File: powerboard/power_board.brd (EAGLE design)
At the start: 149.9 x 86.4 mm, 100 parts, among them Q1 IPP80P03P4L04AKSA1, U1 UWQ-12/20-T48NBS-C, U2 UWE-5/20-Q48NB-C, U3 UWE-3.3/30-Q48NB-C

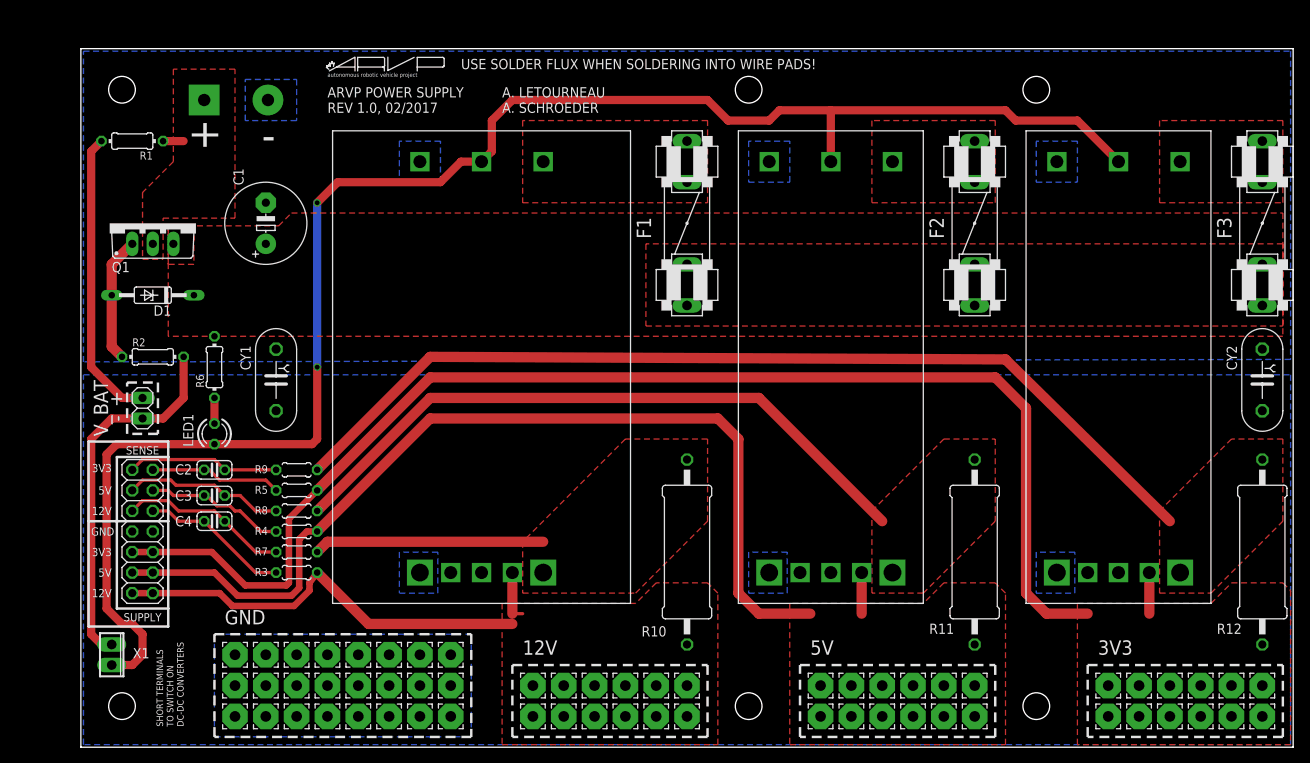
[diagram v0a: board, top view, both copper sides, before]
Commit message: fixed the branch
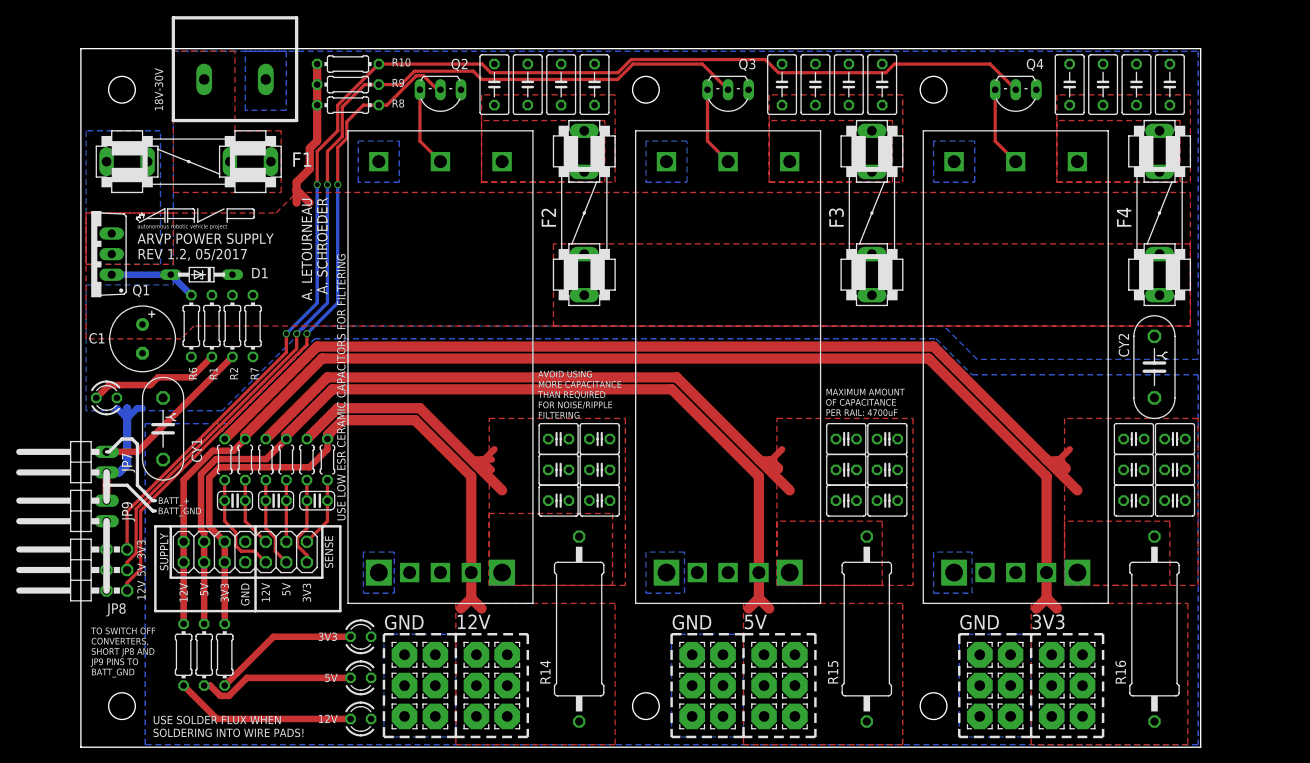
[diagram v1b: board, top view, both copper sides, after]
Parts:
- removed P$1: AND_PWR, ARVP:AND_PWR
- removed PAD37, PAD38, PAD39, PAD40, PAD41, PAD42, PAD43, PAD44, PAD45, PAD46, PAD47, PAD48, PAD49, PAD50, PAD51, PAD52, PAD53, PAD54, PAD55, PAD56, PAD57, PAD58, PAD59, PAD60: WIREPAD3,17/1,3, wirepad:3,17/1,3
- removed U3: UWE-3.3/30-Q48NB-C, New Power Board Library:UWE-100-120W
- removed X1: (no value), con-phoenix-254:2POL254
- added C10, C11, C12, C13, C14, C15, C16, C5, C6, C7, C8, C9: (no value), rcl:C050-035X075
- added C17, C18, C19, C20, C21, C22, C23, C24, C25, C26, C27, C28, C29, C30, C31, C32, C33, C34: (no value), rcl:C025-040X050
- added F4: (no value), special:FUSE1
- added JP10: (no value), pinhead:2X07
- added JP9: (no value), pinhead:1X02/90
- added LED2, LED3, LED4: (no value), led:LED3MM
- added Q2, Q3, Q4: 2N4401TFR, New Power Board Library:TO92-EBC
- added R13: 10, rcl:0204/5
- added R14, R15, R16: 0.004, rcl:0617/22
- added R17, R18, R19: 36k, resistor:0204/7
- added T1: 2_POS_TERMINAL, New Power Board Library:PHOENIX_CONTACT_MKDS_5/2-7.62
- added U4: UWE-12/10-Q48NB-C, New Power Board Library:UWE-100-120W
- C1: value (none) -> 100u; device rcl:E5-10,5 -> rcl:E3,5-8
- D1: value (none) -> BZV10; device diode:DO35Z10 -> diode:DO34Z7
- JP7: device pinhead:1X02 -> pinhead:1X02/90
- JP8: device pinhead:2X07 -> pinhead:2X03/90
- R1: value 1k -> 36k
- R10: value 0.004 -> 10k; device rcl:0617/22 -> resistor:0204/7
- R11, R12: value 0.004 -> 10; device rcl:0617/22 -> rcl:0204/5
- R2: value 100k -> 4.7k
- R6: value 1k -> 2k
- R7: value 10 -> 4.7k; device rcl:0204/5 -> resistor:0204/7
- R8, R9: value 10 -> 10k; device rcl:0204/5 -> resistor:0204/7
- U$1: device frames:DINA5_L -> frames:FRAME_A_L
- U1: value UWQ-12/20-T48NBS-C -> UWE-5/20-Q48NB-C; device New Power Board Library:UWQ-12/20-T48 -> New Power Board Library:UWE-100-120W
- U2: value UWE-5/20-Q48NB-C -> UWE-3.3/30-Q48NB-C
- moved R12 121.2 mm to (54.6, 26.7), turned to 90 degrees
- moved PAD9 92.2 mm to (140.3, 2.54), turned to 90 degrees
- moved R11 90.9 mm to (49.5, 26.7), turned to 90 degrees
- moved PAD18 88.3 mm to (144.1, -1.27), turned to 90 degrees
- moved PAD17 84.8 mm to (144.1, 2.54), turned to 90 degrees
- moved PAD12 80.7 mm to (140.3, -5.08), turned to 90 degrees
- moved R10 73.5 mm to (62.2, 75.6), turned to 0 degrees
- moved PAD7 73.4 mm to (144.1, -5.08), turned to 90 degrees
- moved PAD8 65.5 mm to (140.3, -1.27), turned to 90 degrees
- moved PAD35 64.1 mm to (153.0, -1.27)
- moved PAD36 64.1 mm to (149.2, -1.27)
- moved F1 62.1 mm to (42.5, 63.5), turned to 180 degrees
- moved PAD31 56.6 mm to (153.0, 2.54)
- moved PAD34 56.6 mm to (149.2, -5.08)
- moved PAD10 56.5 mm to (108.6, -1.27)
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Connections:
- removed net N$6: F2.2A, F2.2B, U2.+VIN
- removed net ON/OFF: LED1.K, U1.RC, U2.RC, U3.RC, X1.2
- new net ENABLE_12V: Q2.C, U4.RC
- new net ENABLE_3V3: Q4.C, U2.RC
- new net ENABLE_5V: Q3.C, U1.RC
- new net N$10: LED3.A, R18.1
- new net N$11: LED4.A, R19.1
- new net N$12: C10.1, C15.1, C16.1, C9.1, F4.2A, F4.2B, U2.+VIN
- new net N$3: F1.1A, F1.1B, T1.P$1
- new net N$8: JP8.2, JP8.4, JP8.6, JP9.1
- new net N$9: LED2.A, R17.1
- new net ON/OFF_1: JP8.1, Q2.B, R8.2
- new net ON/OFF_2: JP8.3, Q3.B, R9.2
- new net ON/OFF_3: JP8.5, Q4.B, R10.2
- net 12V+SENSE: now also C17.1, C18.1, C23.1, C24.1, C29.1, C30.1, R14.1, R5.1, U4.+VOUT; no longer R10.1, R7.2, U1.+VOUT
- net 12V-SENSE: now also JP10.5, JP10.6, PAD19.1, PAD20.1, PAD21.1, PAD22.1, PAD23.1, PAD24.1, R13.2, R14.2, R17.2, U4.+SENSE; no longer JP8.1, JP8.2, PAD25.1, PAD26.1, PAD27.1, PAD28.1, PAD29.1, PAD30.1, PAD31.1, PAD32.1, PAD33.1, PAD34.1, PAD35.1, PAD36.1, R10.2, R3.1, U1.+SENSE
- net 3V3+SENSE: now also C21.1, C22.1, C27.1, C28.1, C33.1, C34.1, R16.1, R3.1, U2.+VOUT; no longer R12.1, R9.2, U3.+VOUT
- net 3V3-SENSE: now also JP10.1, JP10.2, PAD31.1, PAD32.1, PAD33.1, PAD34.1, PAD35.1, PAD36.1, R11.2, R16.2, R19.2, U2.+SENSE; no longer JP8.5, JP8.6, PAD49.1, PAD50.1, PAD51.1, PAD52.1, PAD53.1, PAD54.1, PAD55.1, PAD56.1, PAD57.1, PAD58.1, PAD59.1, PAD60.1, R12.2, R5.1, U3.+SENSE
- net 5V+SENSE: now also C19.1, C20.1, C25.1, C26.1, C31.1, C32.1, R15.1, R4.1, U1.+VOUT; no longer R11.1, R8.2, U2.+VOUT
- net 5V-SENSE: now also JP10.3, JP10.4, PAD25.1, PAD26.1, PAD27.1, PAD28.1, PAD29.1, PAD30.1, R12.2, R15.2, R18.2, U1.+SENSE; no longer JP8.3, JP8.4, PAD37.1, PAD38.1, PAD39.1, PAD40.1, PAD41.1, PAD42.1, PAD43.1, PAD44.1, PAD45.1, PAD46.1, PAD47.1, PAD48.1, R11.2, R4.1, U2.+SENSE
- net GND: now also C17.2, C18.2, C19.2, C20.2, C21.2, C22.2, C23.2, C24.2, C25.2, C26.2, C27.2, C28.2, C29.2, C30.2, C31.2, C32.2, C33.2, C34.2, JP10.7, JP10.8, LED2.K, LED3.K, LED4.K, U4.-SENSE, U4.-VOUT; no longer JP8.7, JP8.8, PAD19.1, PAD20.1, PAD21.1, PAD22.1, PAD23.1, PAD24.1, U3.-SENSE, U3.-VOUT
- net J3: now also JP10.9; no longer JP8.9
- net J4: now also JP10.10, R11.1; no longer JP8.10, R7.1
- net J5: now also JP10.11; no longer JP8.11
- net J6: now also JP10.12, R12.1; no longer JP8.12, R8.1
- net J7: now also JP10.13; no longer JP8.13
- net J8: now also JP10.14, R13.1; no longer JP8.14, R9.1
- net N$1: now also R1.1; no longer R6.1
- net N$2: now also JP7.2, R2.2; no longer JP7.1, R1.2
- net N$4: now also R6.1; no longer R2.1
- net N$5: now also C11.1, C12.1, C5.1, C6.1, F2.2A, F2.2B, U4.+VIN; no longer F1.2A, F1.2B, U1.+VIN
- net N$7: now also C13.1, C14.1, C7.1, C8.1, U1.+VIN; no longer U3.+VIN
- net V+: now also F4.1A, F4.1B, R1.2, R10.1, R2.1, R7.1, R8.1, R9.1; no longer F1.1A, F1.1B, R6.2
- net V-: now also C10.2, C11.2, C12.2, C13.2, C14.2, C15.2, C16.2, C5.2, C6.2, C7.2, C8.2, C9.2, JP7.1, JP9.2, LED1.K, Q2.E, Q3.E, Q4.E, R6.2, R7.2, T1.P$2, U4.-VIN; no longer JP7.2, P$1.GND, R2.2, U3.-VIN, X1.1
- net VBAT+: now also F1.2A, F1.2B; no longer P$1.PWR, R1.1
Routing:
- net ON/OFF: track 204.8 -> 0.00 mm, vias 2 -> 0
- net ON/OFF_3: track 0.00 -> 155.2 mm, vias 0 -> 2
- net ON/OFF_2: track 0.00 -> 120.3 mm, vias 0 -> 2
- net ON/OFF_1: track 0.00 -> 83.9 mm, vias 0 -> 2
- net V-: track 45.8 -> 17.6 mm
- net N$11: track 0.00 -> 22.3 mm
- net V+: track 0.00 -> 20.4 mm
- net N$10: track 0.00 -> 19.5 mm
- net N$9: track 0.00 -> 18.1 mm
- net 12V-SENSE: track 59.0 -> 76.8 mm
- net N$2: track 36.4 -> 20.4 mm
- net N$1: track 3.18 -> 16.4 mm
- net J4: track 20.9 -> 8.67 mm
- net J6: track 19.9 -> 7.62 mm
- net J8: track 18.8 -> 8.67 mm
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- added copper zone on layer 1, net N$12
- added copper zone on layer 1, net N$3
- added copper zone on layer 16, net VBAT+
- removed copper zone on layer 1, net N$6
- removed copper zone on layer 1, net VBAT+
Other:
- board size 149.9 x 86.4 mm -> 138.4 x 86.4 mm
- board text added: "18V-30V"
- board text added: "AVOID USING"
- board text added: "BATT_+"
- board text added: "BATT_GND"
- board text added: "CONVERTERS,"
- board text added: "FILTERING"
- board text added: "FOR NOISE/RIPPLE"
- board text added: "JP9 PINS TO"
- board text added: "MAXIMUM AMOUNT"
- board text added: "MORE CAPACITANCE"
- board text added: "OF CAPACITANCE"
- board text added: "PER RAIL: 4700uF"
- board text added: "REV 1.2, 05/2017"
- board text added: "SHORT JP8 AND"
- board text added: "SOLDERING INTO WIRE PADS!"
- board text added: "THAN REQUIRED"
- board text added: "TO SWITCH OFF"
- board text added: "USE LOW ESR CERAMIC CAPACITORS FOR FILTERING"
- board text added: "USE SOLDER FLUX WHEN"
- board text added: "UWE-12/10-Q48NB-C"
- board text added: "UWE-3.3/30-Q48NB-C"
- board text added: "UWE-5/20-Q48NB-C"
- board text removed: "DC-DC CONVERTERS"
- board text removed: "REV 1.0, 02/2017"
- board text removed: "SHORT TERMINALS"
- board text removed: "TO SWITCH ON"
- board text removed: "USE SOLDER FLUX WHEN SOLDERING INTO WIRE PADS!"
- board text removed: "V_BAT"
